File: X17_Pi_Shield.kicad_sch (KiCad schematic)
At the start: 0 parts

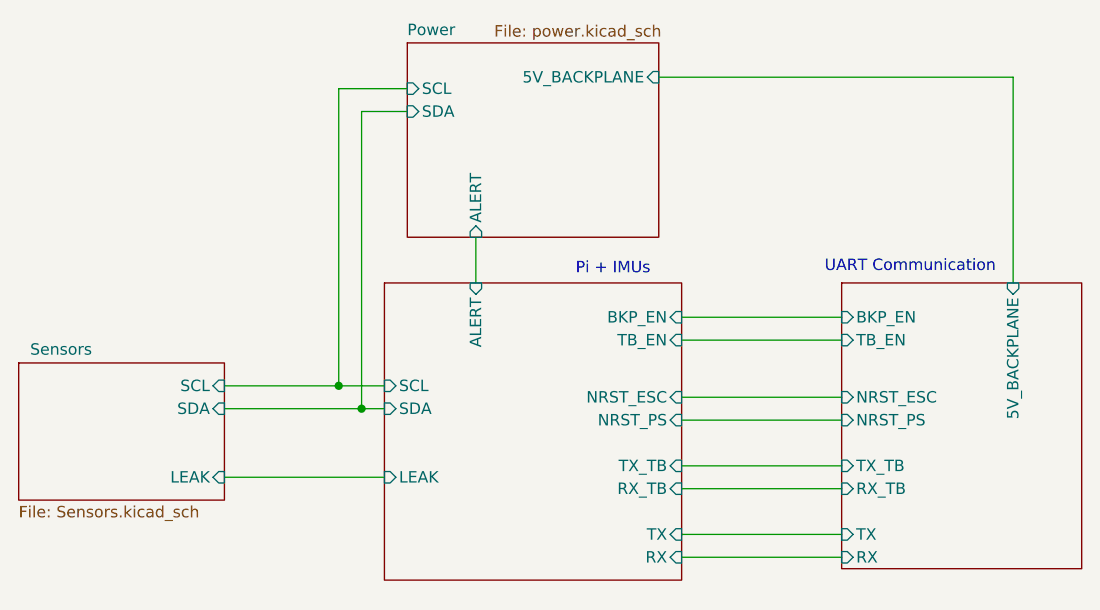
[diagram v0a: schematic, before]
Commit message: Finalized Footprints
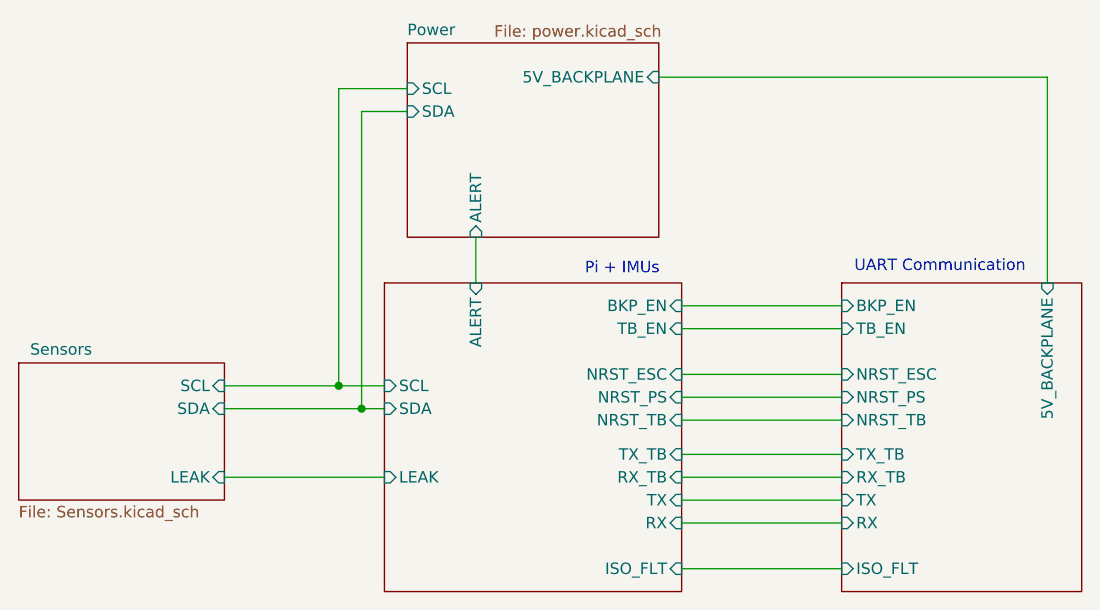
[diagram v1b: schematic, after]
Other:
- sheet Pi + IMU ports: added ISO_FLT, NRST_TB; removed none
- sheet UART ports: added ISO_FLT, NRST_TB; removed none
